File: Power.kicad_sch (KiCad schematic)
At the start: 20 parts, among them Q1 SIS412DN-T1-GE3, Q2 SIS412DN-T1-GE3, SW2 OS102011MA1Q, U10 MCP1703Ax-330xxDB, U14 LTC4365TS8

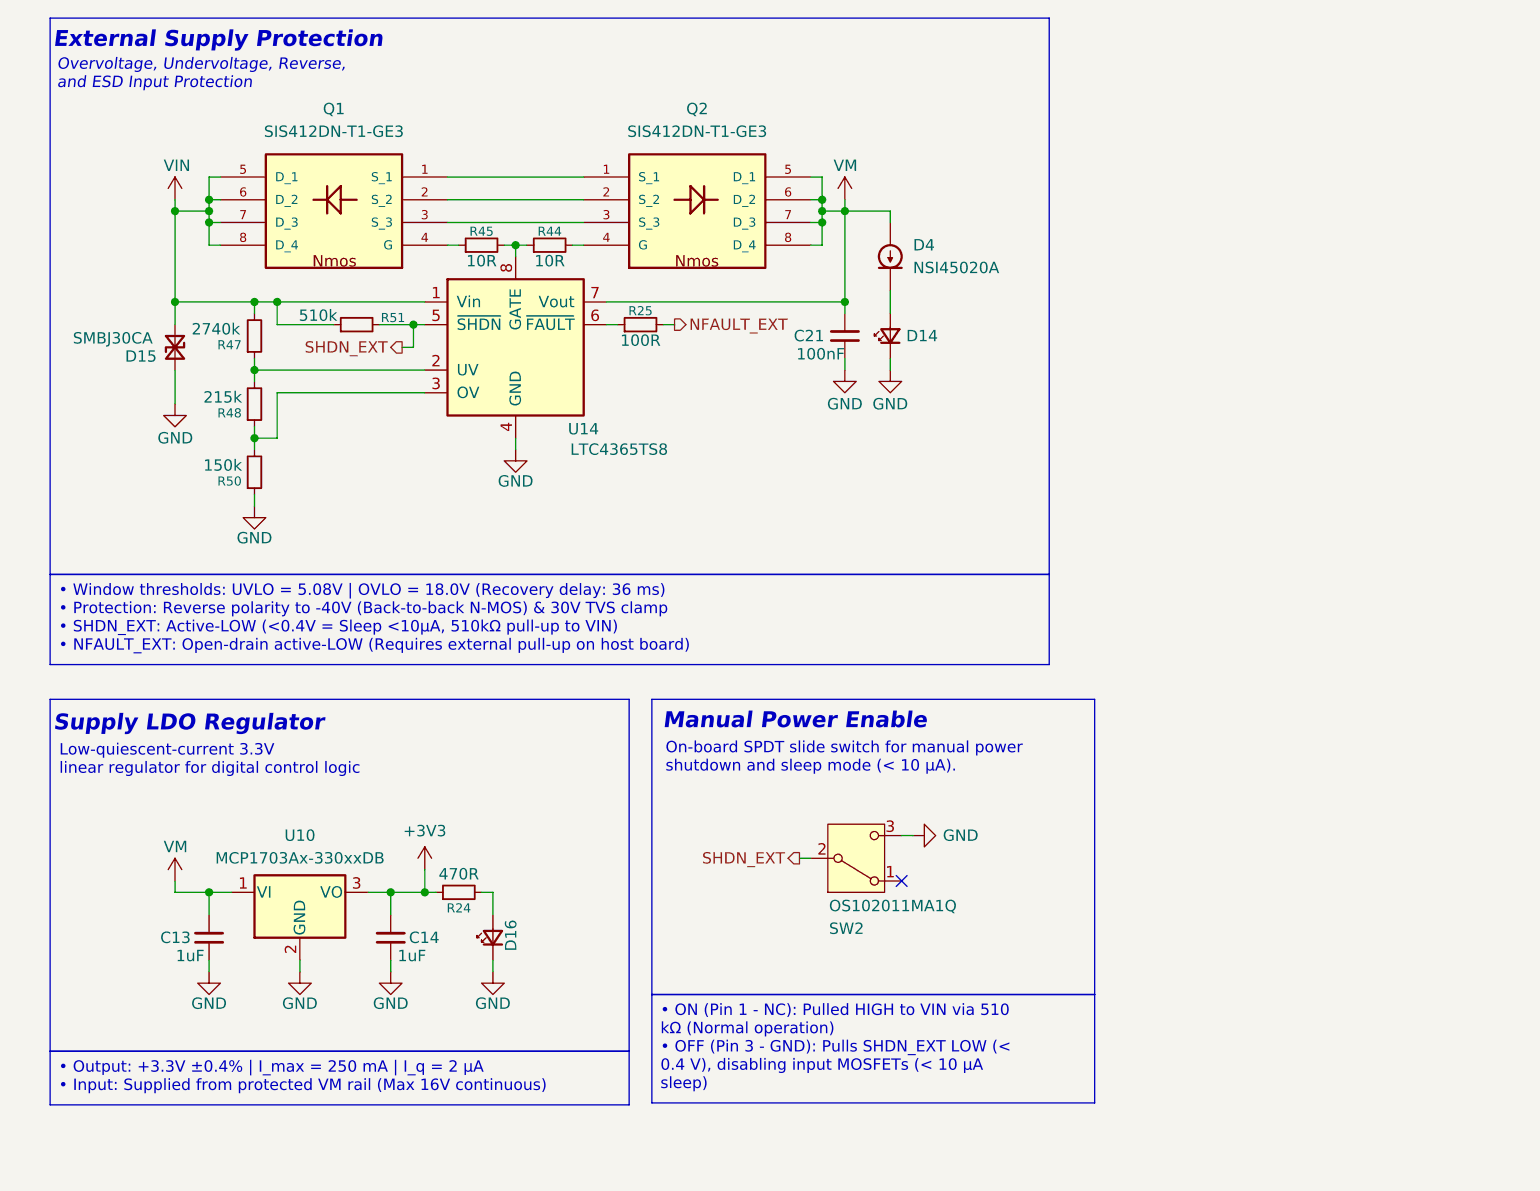
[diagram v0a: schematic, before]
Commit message: fix: fix some errors in shematic
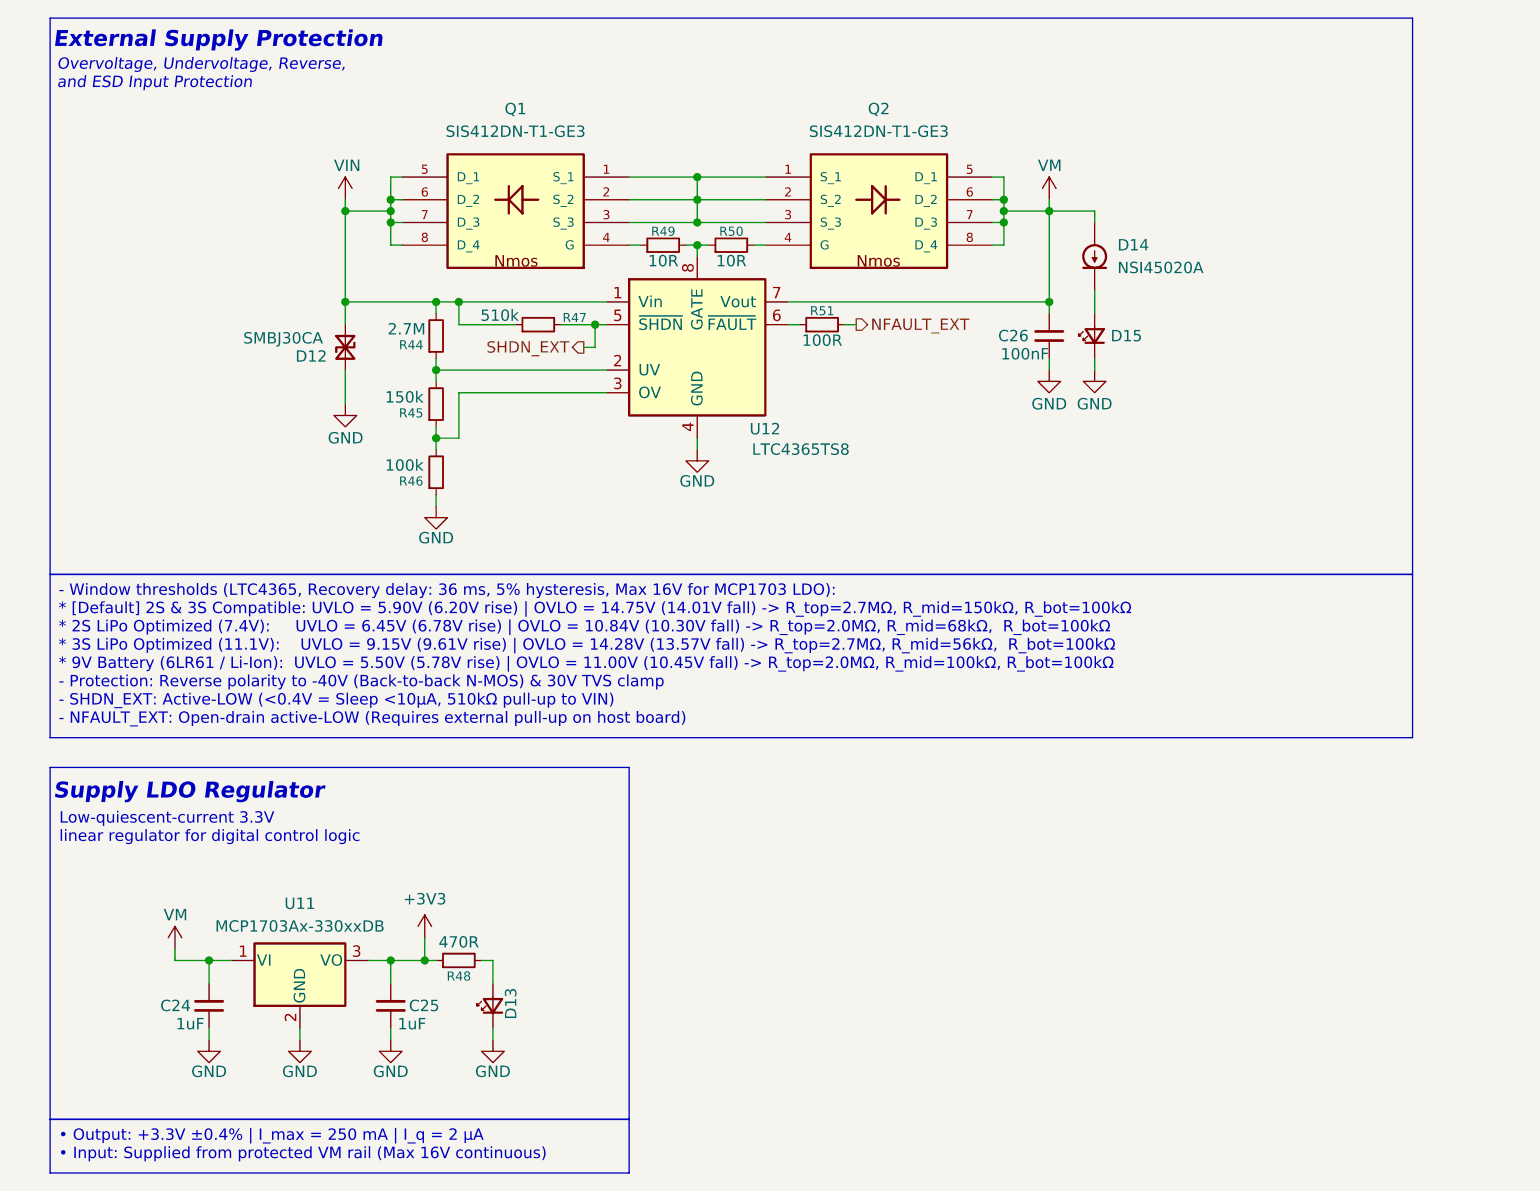
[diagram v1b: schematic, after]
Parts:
- removed SW2: OS102011MA1Q, Button_Switch_THT:SW_Slide_SPDT_Angled_CK_OS102011MA1Q, symbol Switch:SW_SPDT
- Q1, Q2: footprint SIS412DN-T1-GE3:POWERPAK-1212-8 -> KineticCore:POWERPAK-1212-8
- R44: renamed from R47; value 2740k -> 2.7M
- R45: renamed from R48; value 215k -> 150k
- R46: renamed from R50; value 150k -> 100k
- renumbered C13 to C24, C14 to C25, C21 to C26, D15 to D12, D16 to D13, D4 to D14, D14 to D15, R51 to R47, R24 to R48, R45 to R49, R44 to R50, R25 to R51, U10 to U11, U14 to U12
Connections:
- net at Q1.1 (S_1), Q2.1 (S_1): now also Q1.2 (S_2), Q1.3 (S_3), Q2.2 (S_2), Q2.3 (S_3)
- no-connect marks 1 -> 0
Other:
- note removed: "Manual Power Enable"
- note removed: "On-board SPDT slide switch for manual power shutdown and sleep mode (< 10 µA)."
- moved on the sheet: C24, C25, C26, D12, D13, D14, D15, Q1, Q2, R44, R45, R46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
